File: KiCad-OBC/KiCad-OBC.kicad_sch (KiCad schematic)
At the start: 1 part

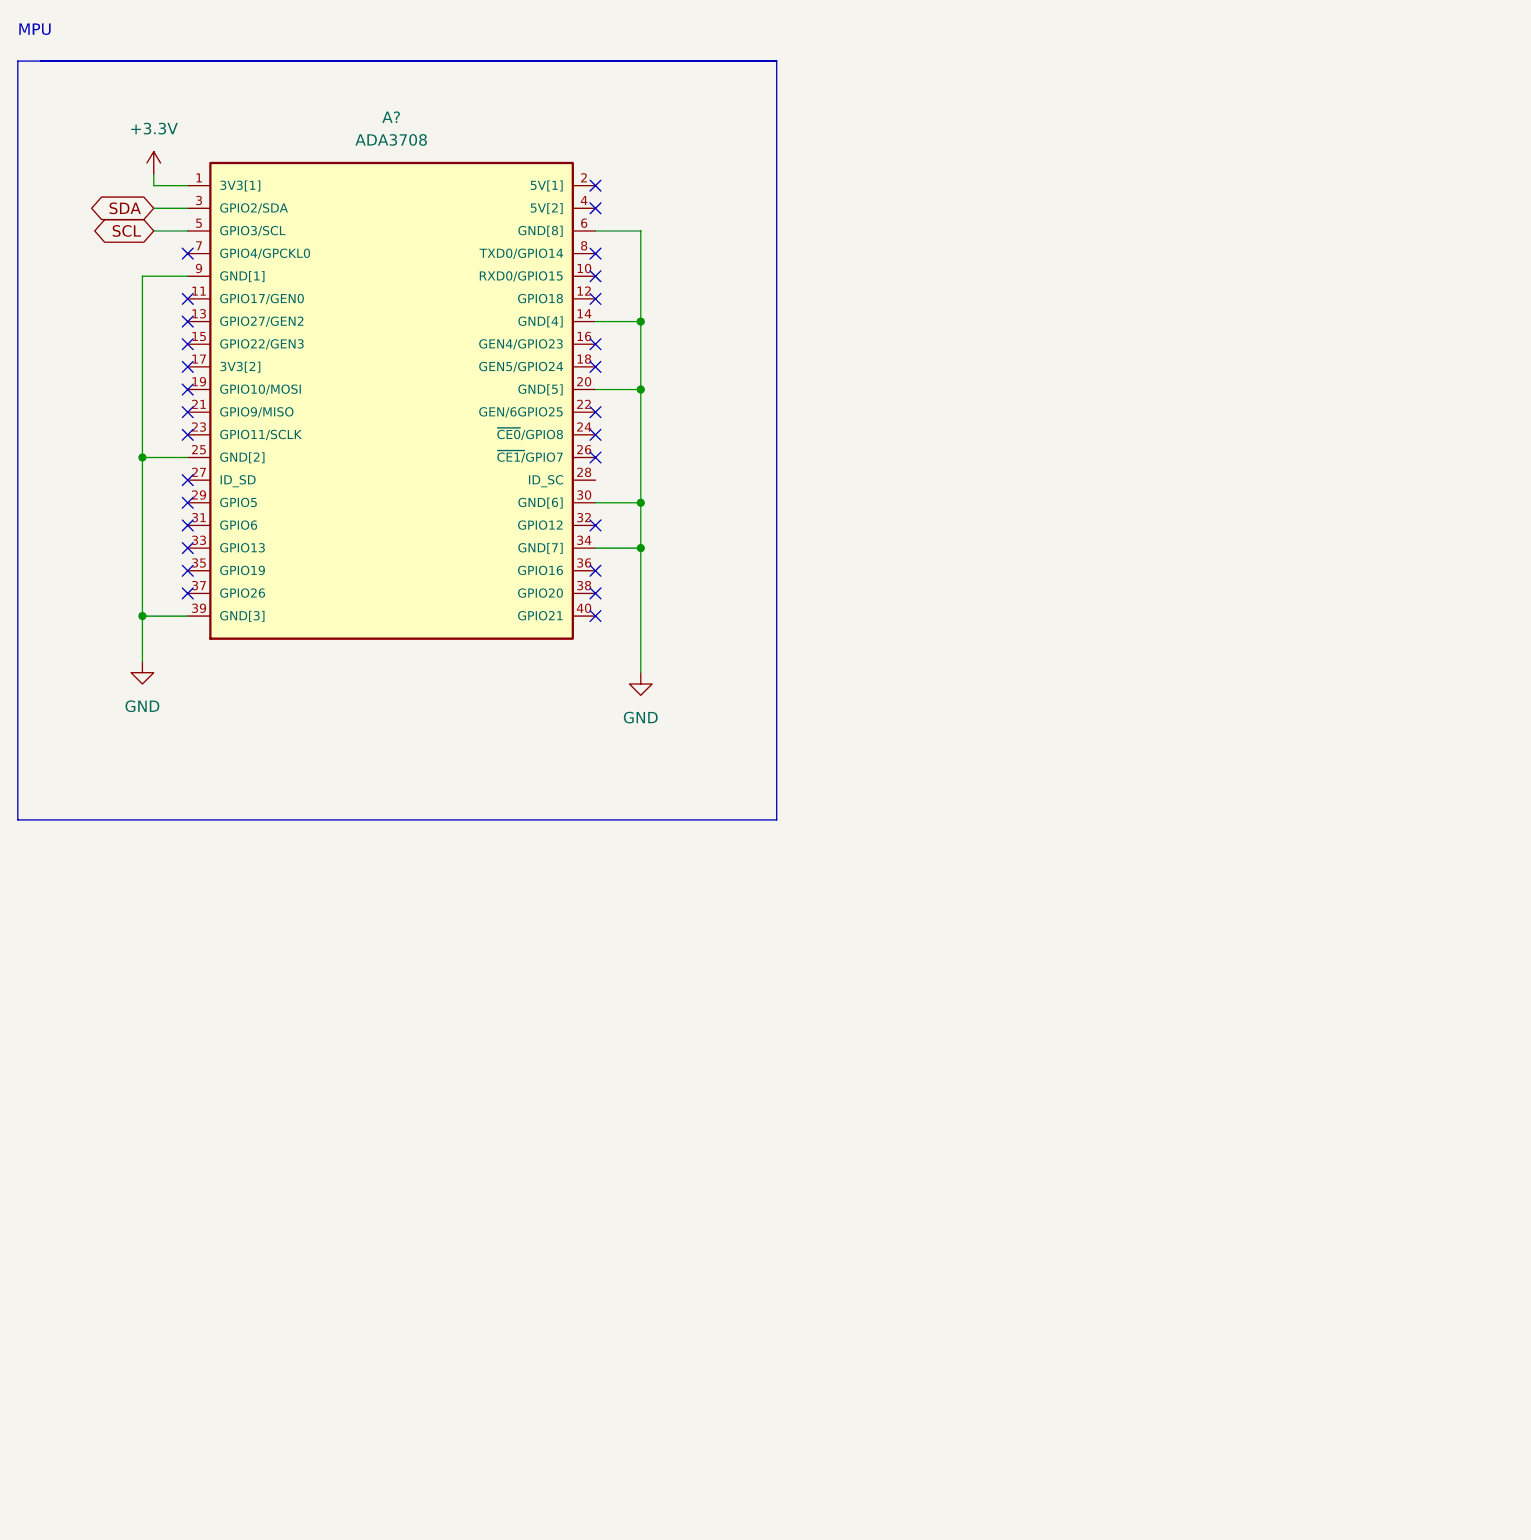
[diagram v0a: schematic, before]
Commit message: schematics finished
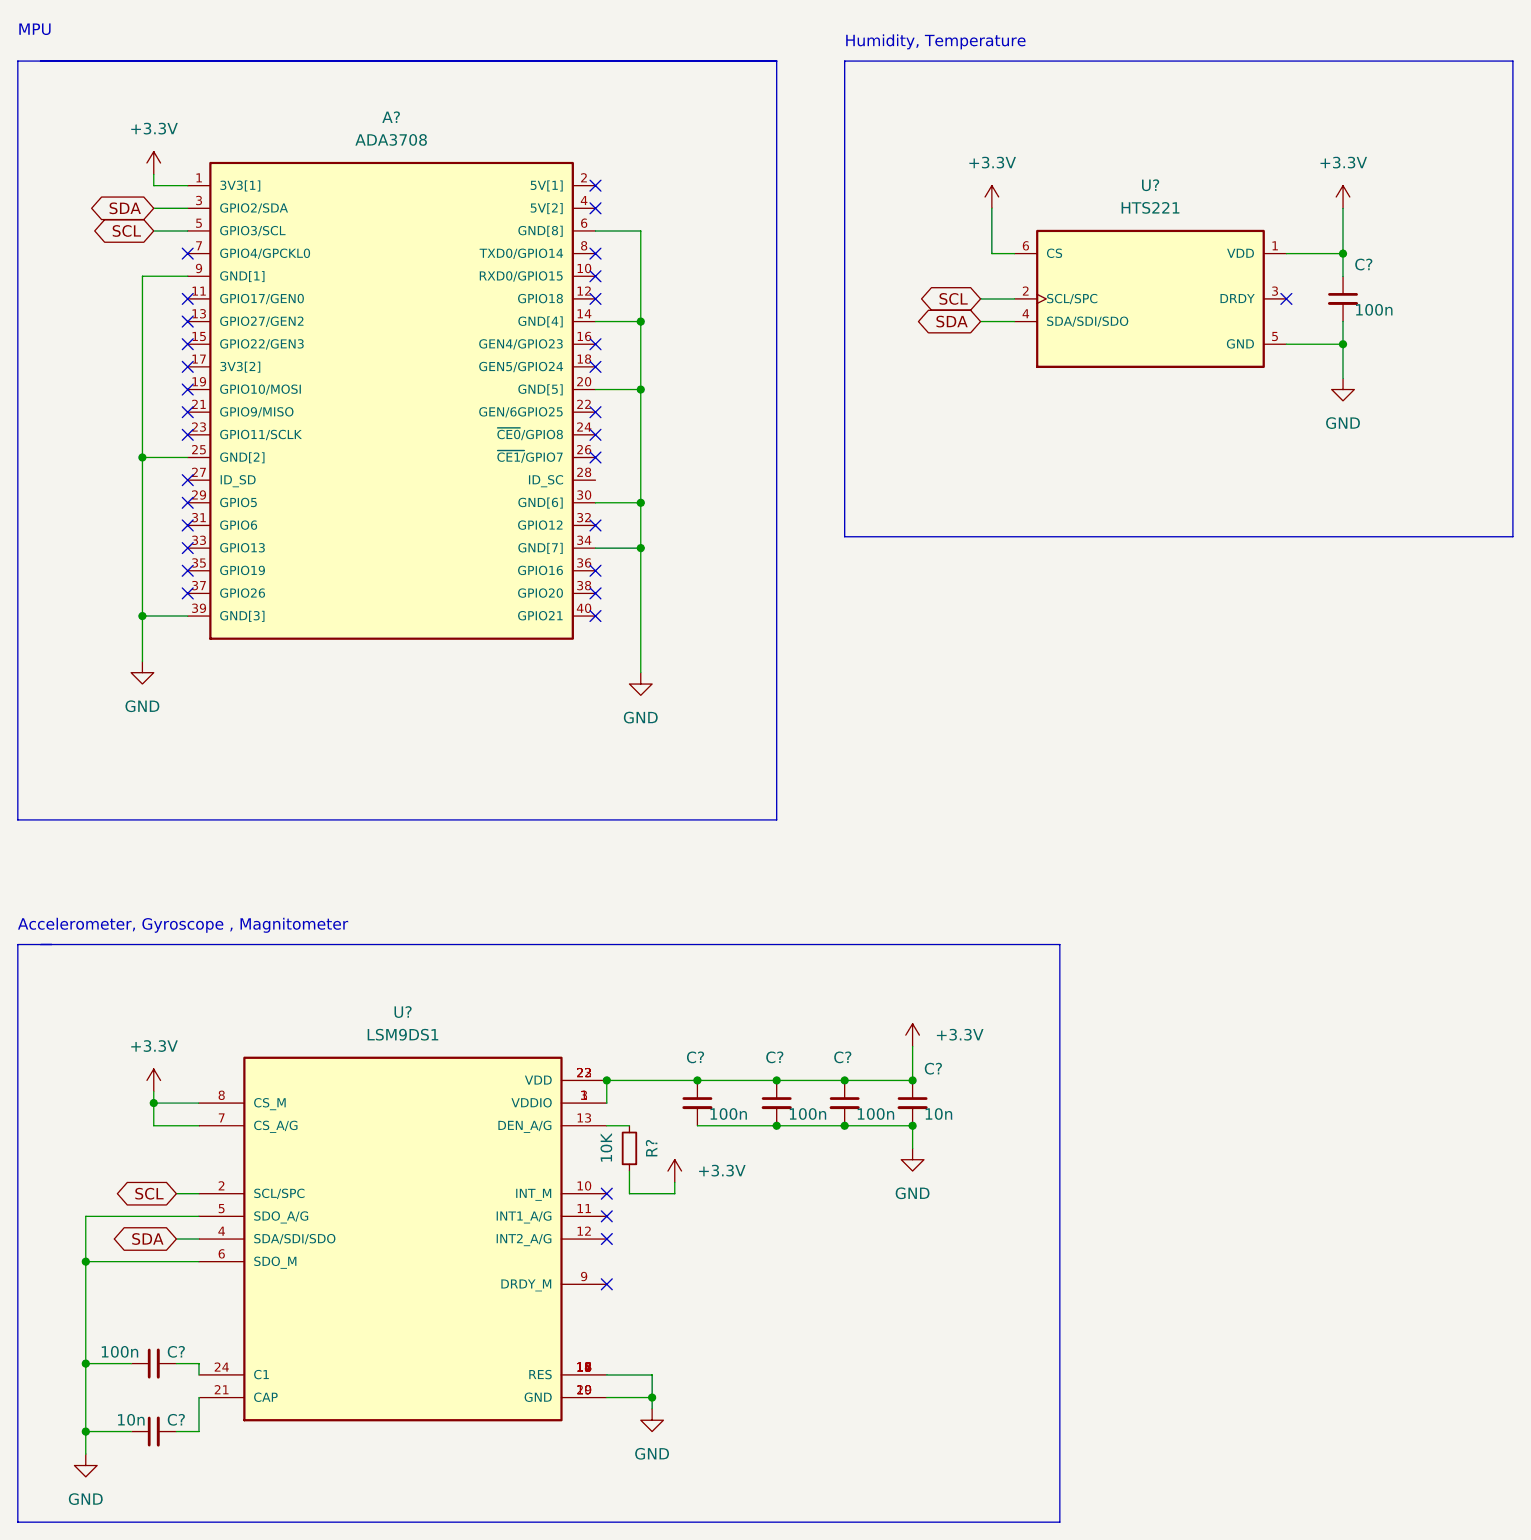
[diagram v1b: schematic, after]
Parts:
- added C? (x5): 100n, symbol Device:C_Small
- added C? (x2): 10n, symbol Device:C_Small
- added R?: 10K, symbol Device:R_Small
- added U?: HTS221, XDCR_HTS221, symbol OBC:HTS221
- added U?: LSM9DS1, PQFN24P43_350X300X102L35X23N, symbol OBC:LSM9DS1
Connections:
- net +3V3: now also C?.1, C?.1, C?.1, C?.1, C?.1, R?.1, U?.1 (VDD), U?.1 (VDDIO), U?.22 (VDD), U?.23 (VDD), U?.3 (VDDIO), U?.6 (CS), U?.7 (CS_A/G), U?.8 (CS_M)
- net GND: now also C?.1, C?.1, C?.2, C?.2, C?.2, C?.2, C?.2, U?.14 (RES), U?.15 (RES), U?.16 (RES), U?.17 (RES), U?.18 (RES), U?.19 (GND), U?.20 (GND), U?.5 (GND), U?.5 (SDO_A/G), U?.6 (SDO_M)
- net SCL: now also U?.2 (SCL/SPC), U?.2 (SCL/SPC)
- net SDA: now also U?.4 (SDA/SDI/SDO), U?.4 (SDA/SDI/SDO)
- new net: C?.2, U?.24 (C1)
- new net: R?.2, U?.13 (DEN_A/G)
- new net: C?.2, U?.21 (CAP)
- no-connect marks 28 -> 33
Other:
- note added: "Accelerometer, Gyroscope , Magnitometer"
- note added: "Humidity, Temperature"

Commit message: start obc again with new place
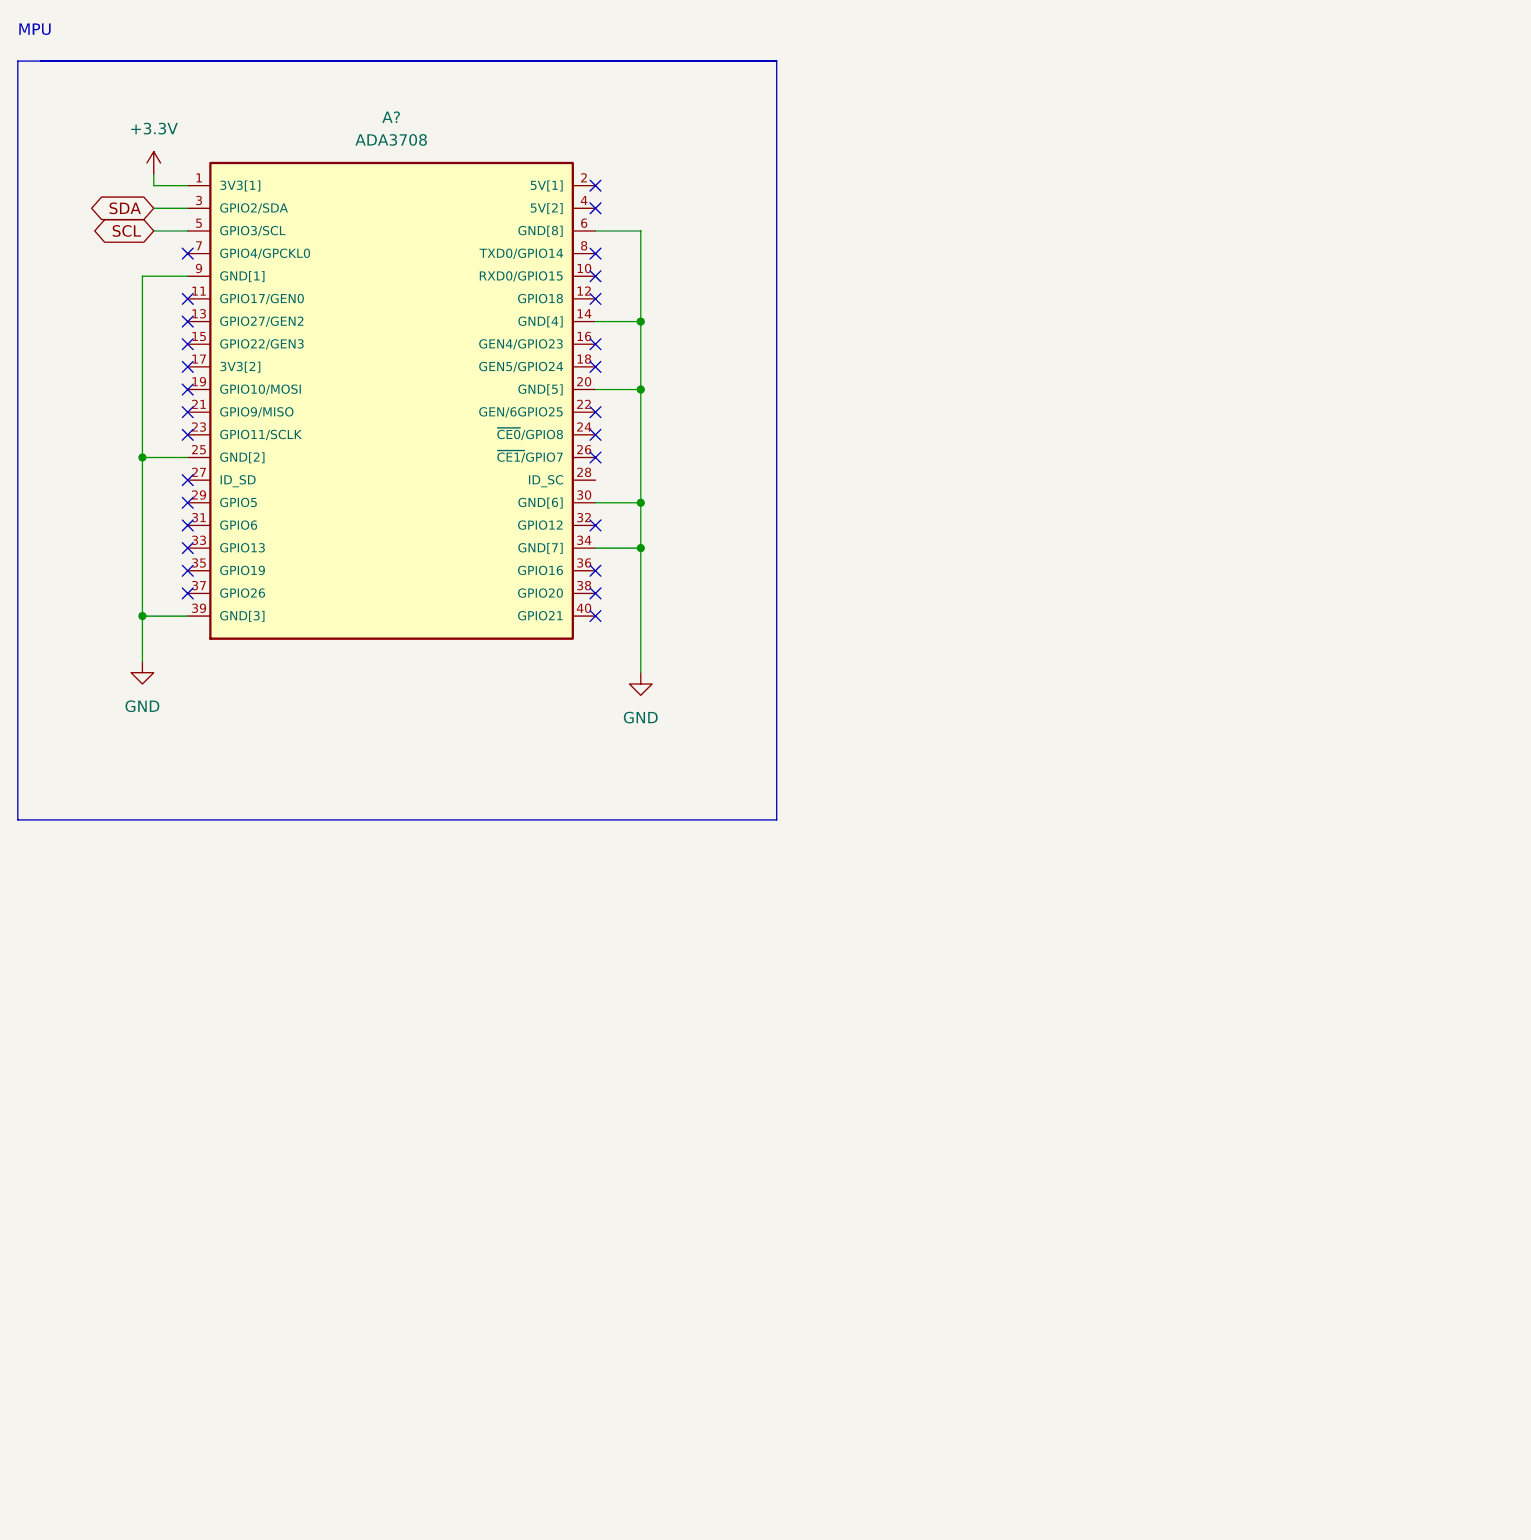
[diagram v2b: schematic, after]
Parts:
- removed C? (x5): 100n, symbol Device:C_Small
- removed C? (x2): 10n, symbol Device:C_Small
- removed R?: 10K, symbol Device:R_Small
- removed U?: HTS221, XDCR_HTS221, symbol OBC:HTS221
- removed U?: LSM9DS1, PQFN24P43_350X300X102L35X23N, symbol OBC:LSM9DS1
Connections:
- no-connect marks 33 -> 28
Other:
- note removed: "Accelerometer, Gyroscope , Magnitometer"
- note removed: "Humidity, Temperature"
